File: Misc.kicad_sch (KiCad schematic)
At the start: 18 parts, among them J3 Conn_02x08_Odd_Even, J4 BM04B-SURS-TFLFSN, J5 Conn_02x04_Odd_Even, J6 Conn_02x04_Odd_Even, J7 Conn_01x05, J8 Conn_01x04, U5 SN65HVD232QDRQ1

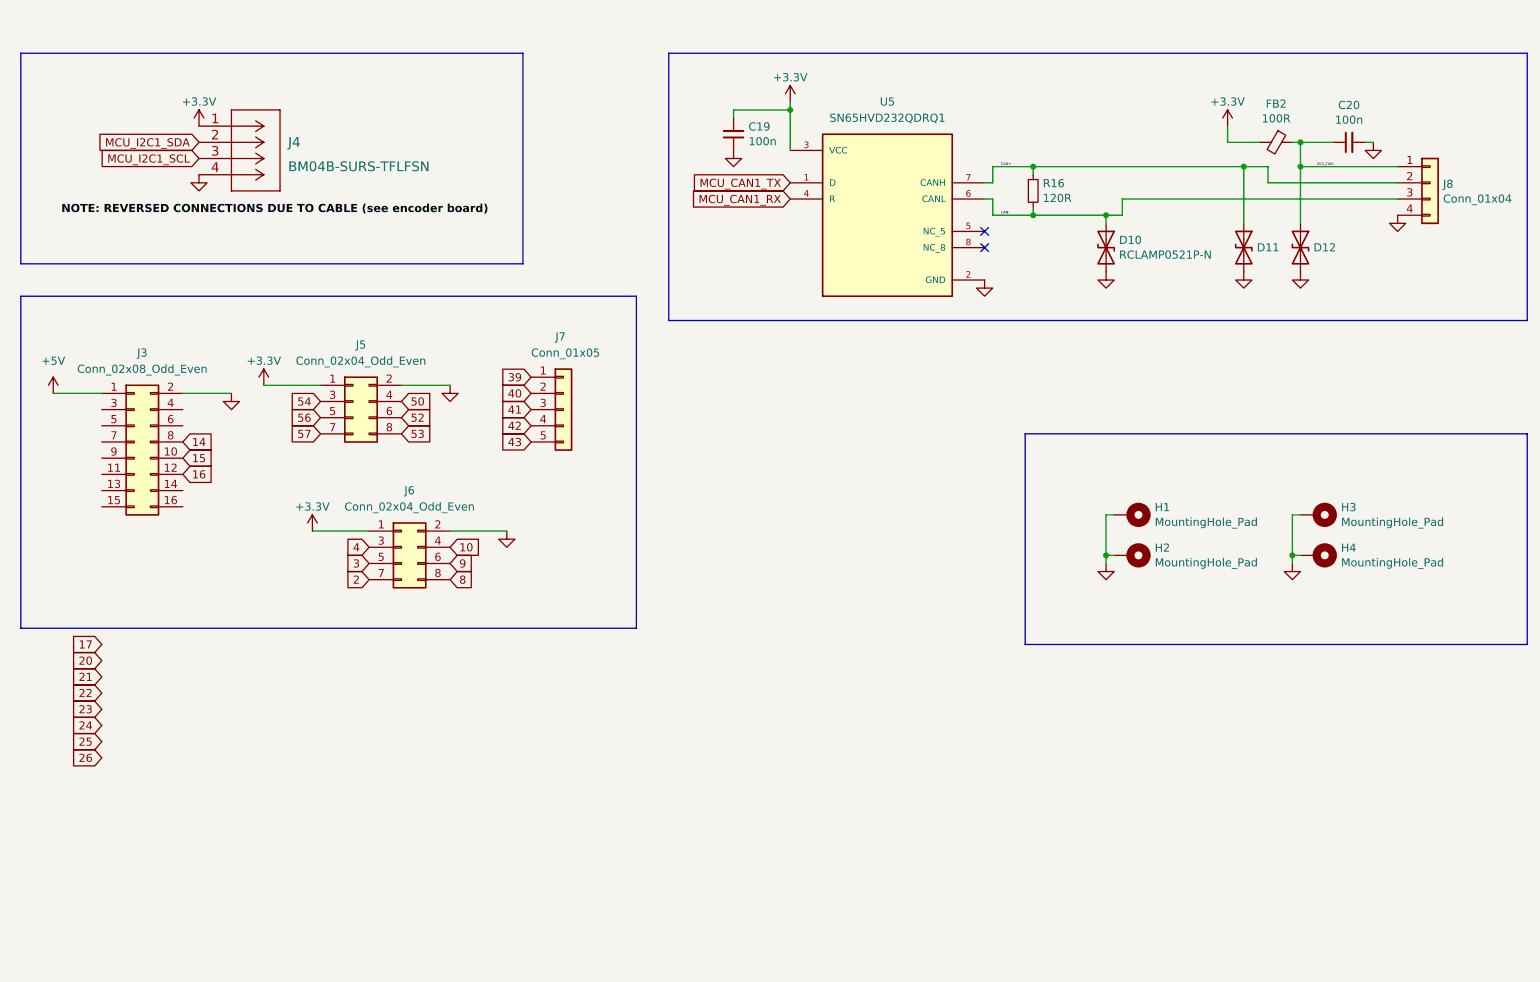
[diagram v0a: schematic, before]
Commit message: sdignionsrg
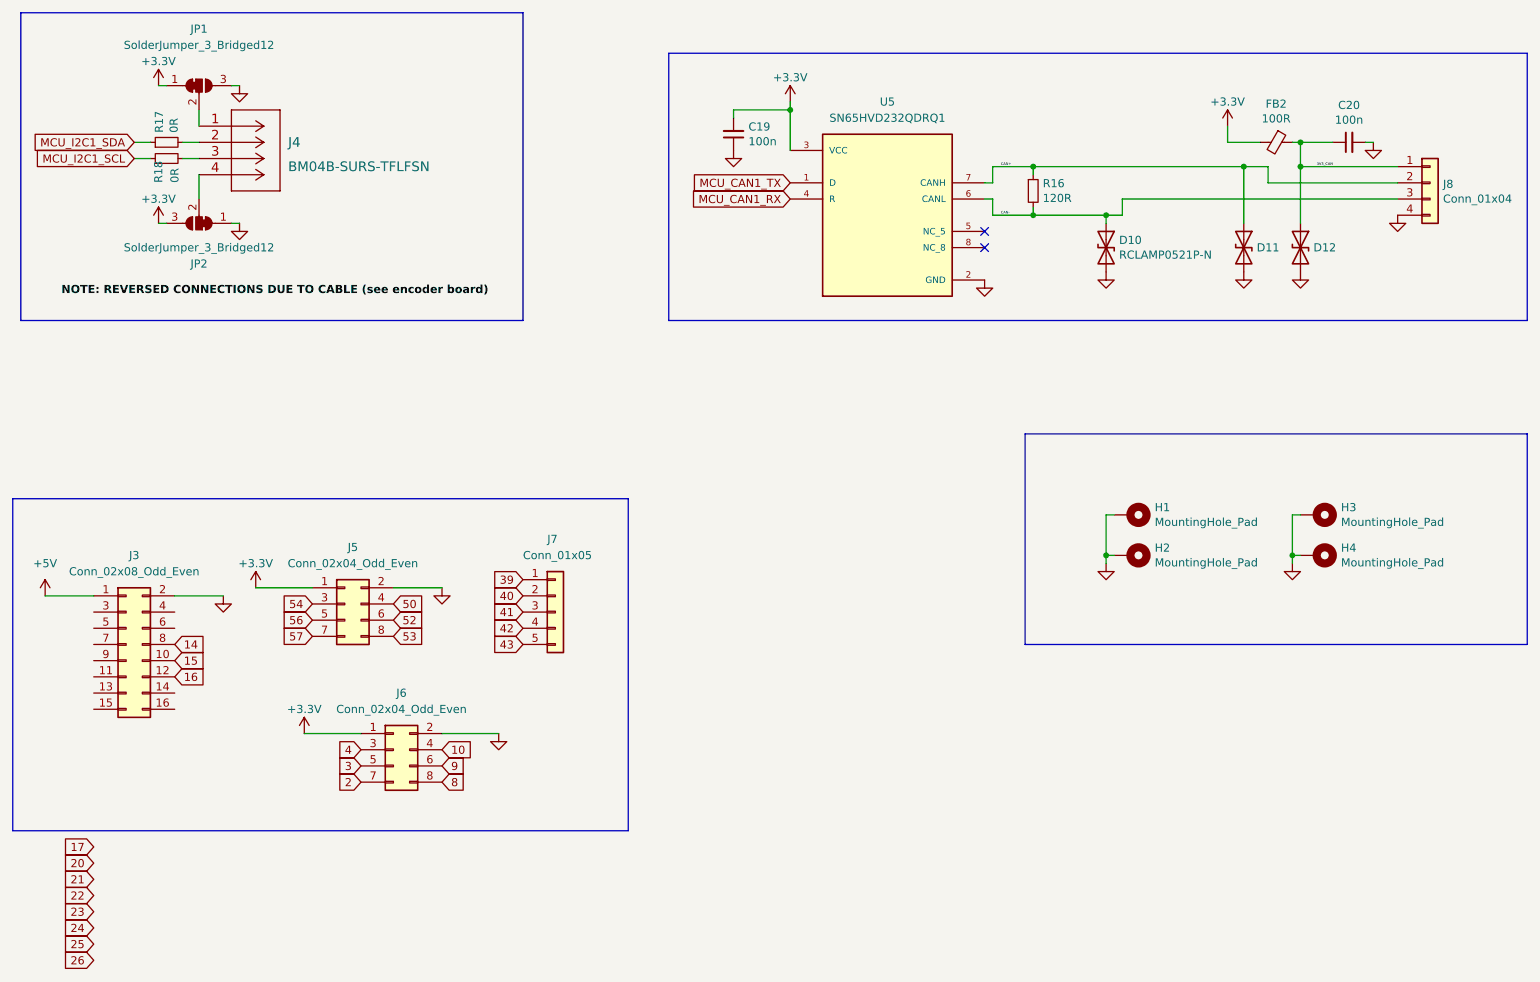
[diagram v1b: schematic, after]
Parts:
- added JP1, JP2: SolderJumper_3_Bridged12, Jumper:SolderJumper-3_P1.3mm_Bridged12_Pad1.0x1.5mm, symbol Jumper:SolderJumper_3_Bridged12
- added R17, R18: 0R, Resistor_SMD:R_0402_1005Metric, symbol Device:R_Small
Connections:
- net +3V3: now also JP1.1 (A), JP2.3 (B); no longer J4.1
- net GND: now also JP1.3 (B), JP2.1 (A); no longer J4.4
- net MCU_I2C1_SCL: now also R18.1; no longer J4.3
- net MCU_I2C1_SDA: now also R17.1; no longer J4.2
- new net: J4.1, JP1.2 (C)
- new net: J4.4, JP2.2 (C)
- new net: J4.2, R17.2
- new net: J4.3, R18.2
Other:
- moved on the sheet: J3, J5, J6, J7
